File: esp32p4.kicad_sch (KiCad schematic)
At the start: 63 parts, among them Q5 AO3400 (A09T), Q6 AO3400 (A09T), U13 W25Q128JVS, U3 TLV62569DBV, U7 CH340K, U8 ESP32-P4, Y3 40MHz

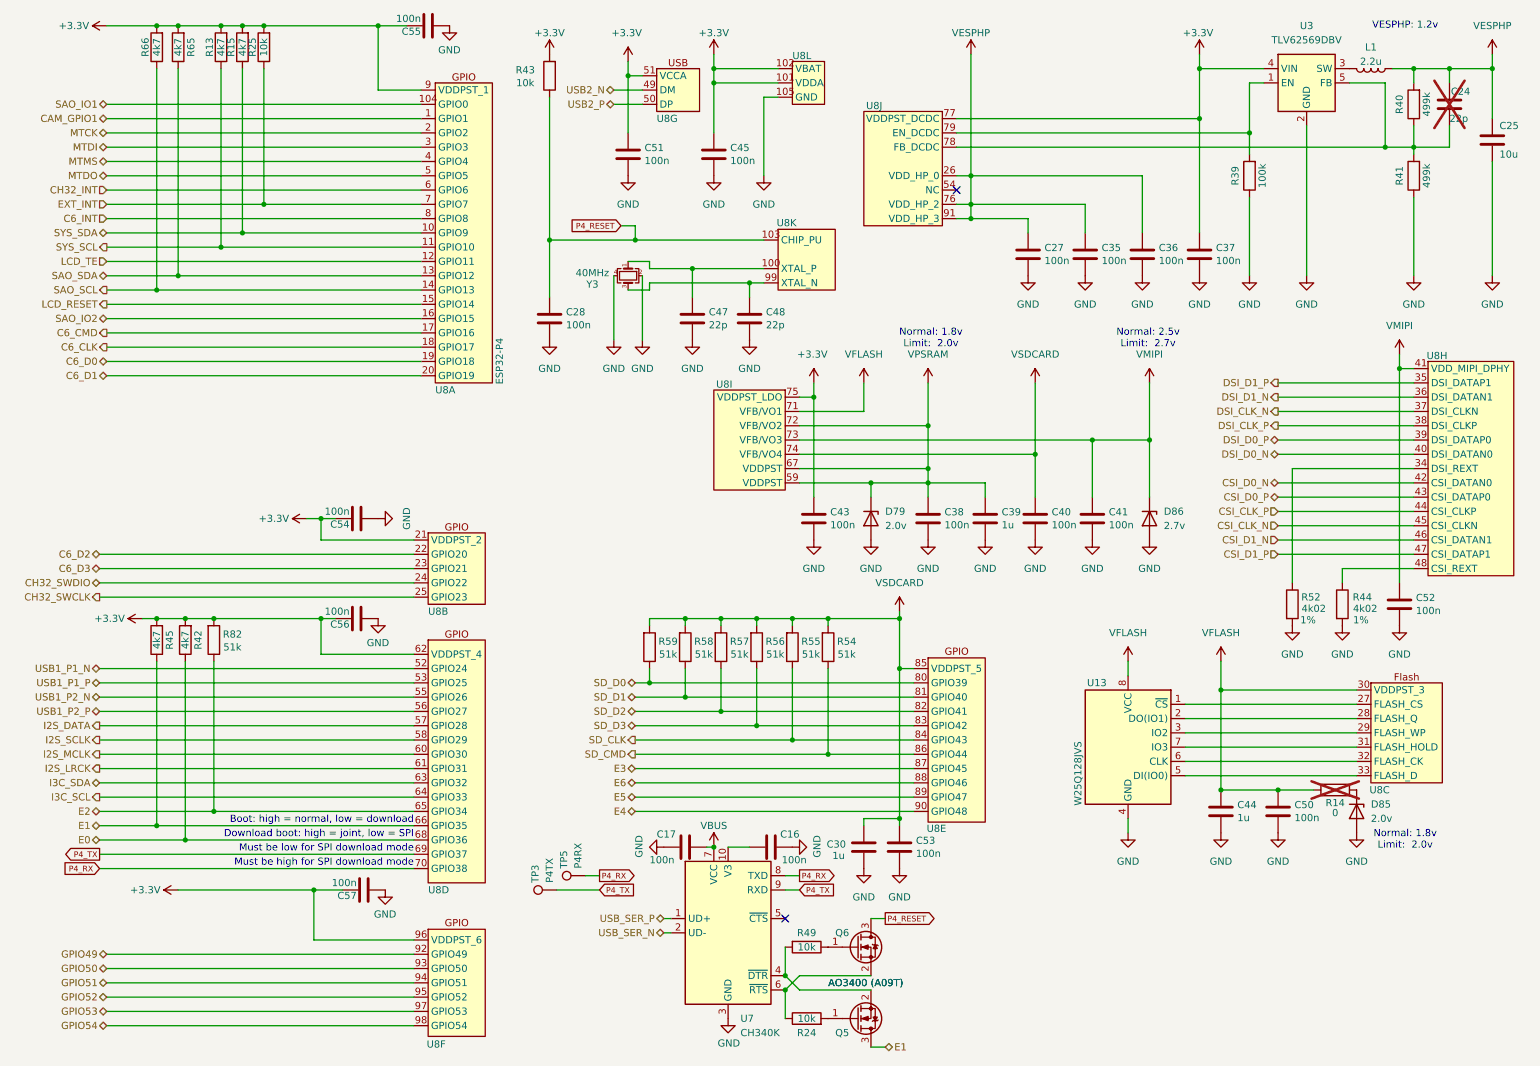
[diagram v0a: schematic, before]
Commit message: Add 1.5k pull-up to D+ of C6, remove logos, add JTAG connector, fix SAO pinout
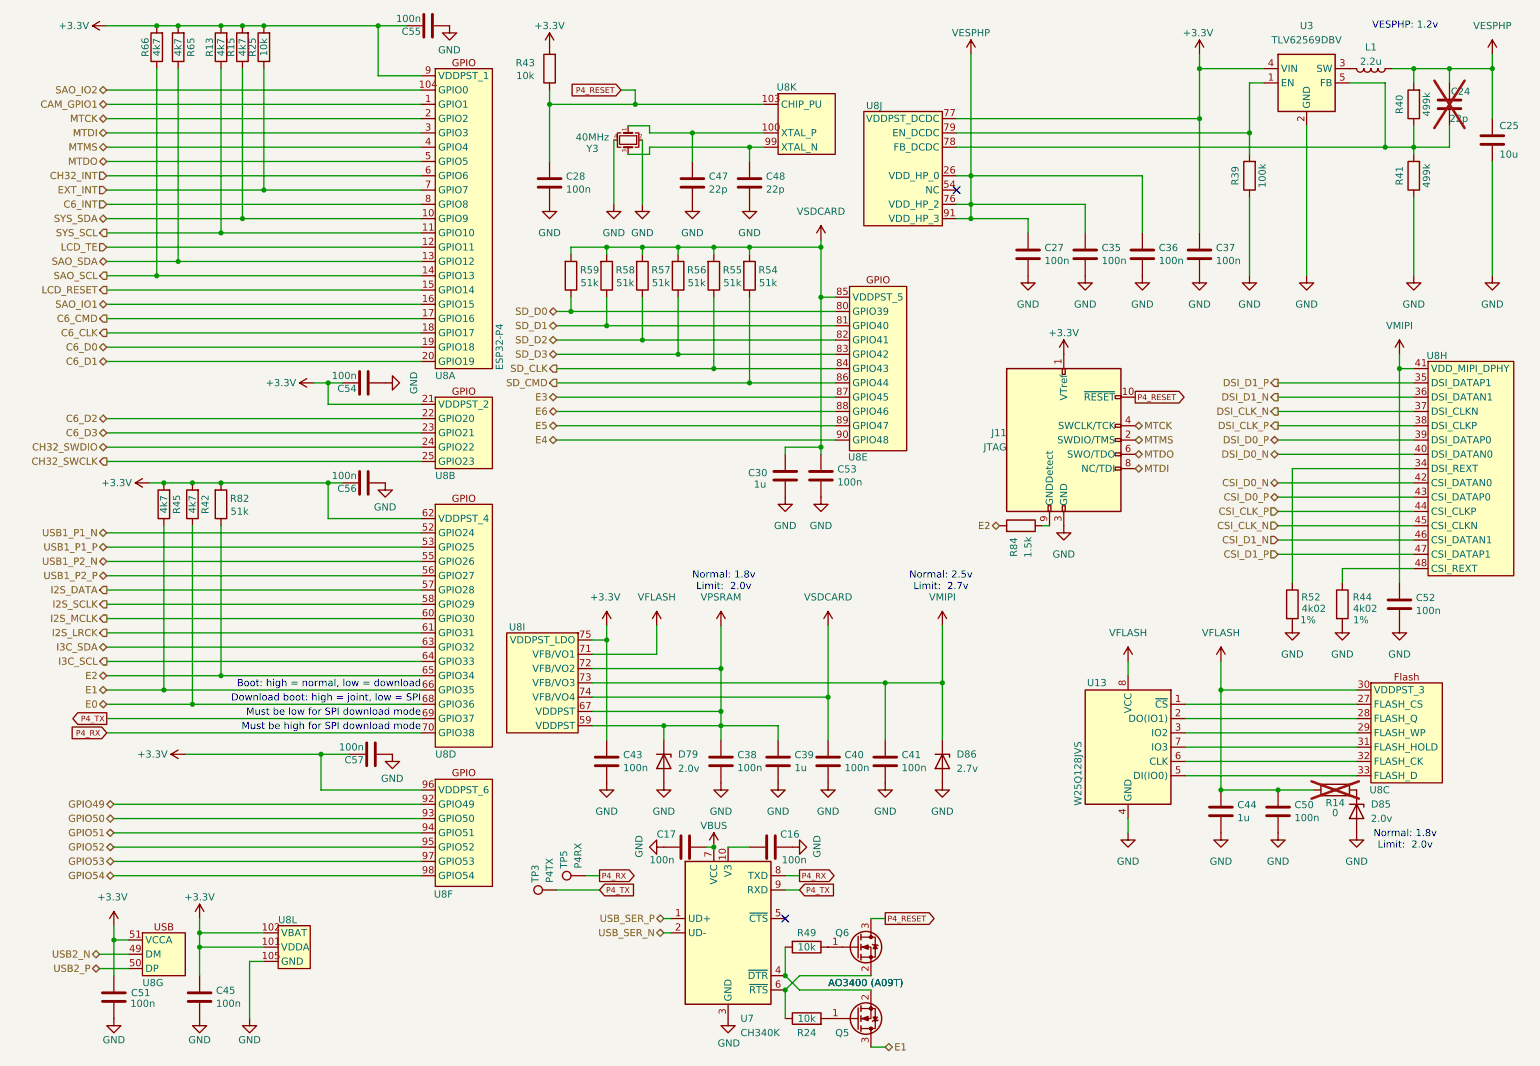
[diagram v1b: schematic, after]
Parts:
- added J11: JTAG, Connector_PinHeader_1.27mm:PinHeader_2x05_P1.27mm_Vertical_SMD, symbol Connector:Conn_ARM_JTAG_SWD_10
- added R84: 1.5k, Resistor_SMD:R_0402_1005Metric, symbol symbols:R
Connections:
- net +3.3V: now also J11.1 (VTref)
- net E2: now also R84.2
- net GND: now also J11.3 (GND), J11.5 (GND)
- net MTCK: now also J11.4 (SWCLK/TCK)
- net MTDI: now also J11.8 (NC/TDI)
- net MTDO: now also J11.6 (SWO/TDO)
- net MTMS: now also J11.2 (SWDIO/TMS)
- net P4_RESET: now also J11.10 (~{RESET})
- net SAO_IO1: now also U8.16 (GPIO15); no longer U8.104 (GPIO0)
- net SAO_IO2: now also U8.104 (GPIO0); no longer U8.16 (GPIO15)
- new net: J11.9 (GNDDetect), R84.1
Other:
- moved on the sheet: C28, C30, C38, C39, C40, C41, C43, C45, C47, C48, C51, C53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

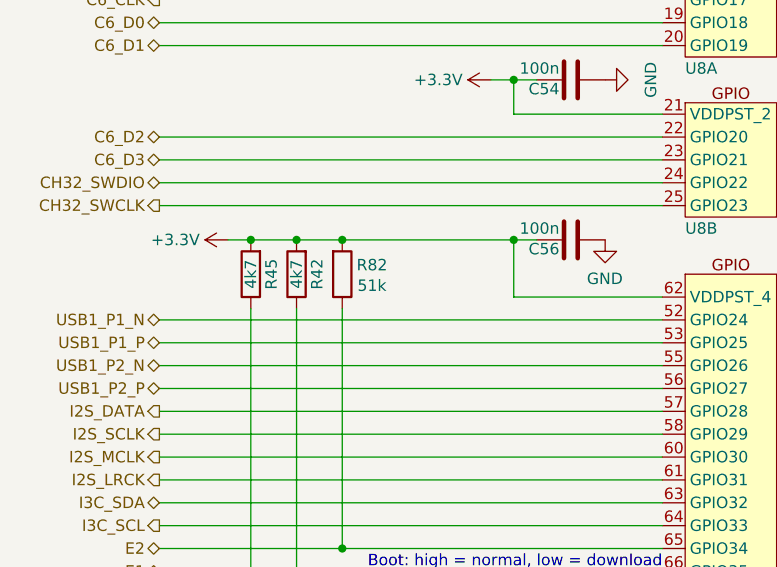
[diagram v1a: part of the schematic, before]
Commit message: Made more space around the D87, smooth curve LORA antenna.
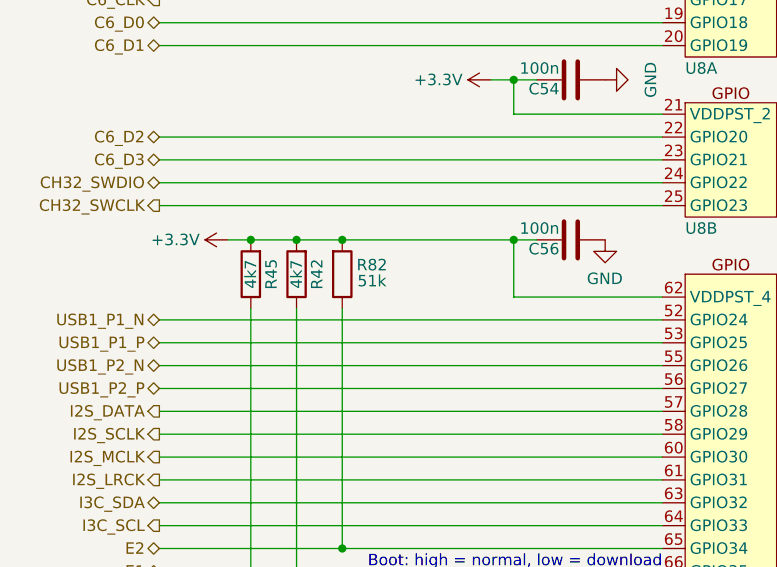
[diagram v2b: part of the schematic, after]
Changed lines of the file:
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@@
 		)
 		(property "Value" "51k"
-			(at 51.562 101.6 0)
+			(at 51.562 101.092 0)
 			(effects
 				(font
